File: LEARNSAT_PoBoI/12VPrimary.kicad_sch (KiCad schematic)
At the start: 17 parts, among them Q201 SI7164DP-T1-GE3, U201 INA219AIDCNR, U202 LTC4231IUD-2#TRPBF

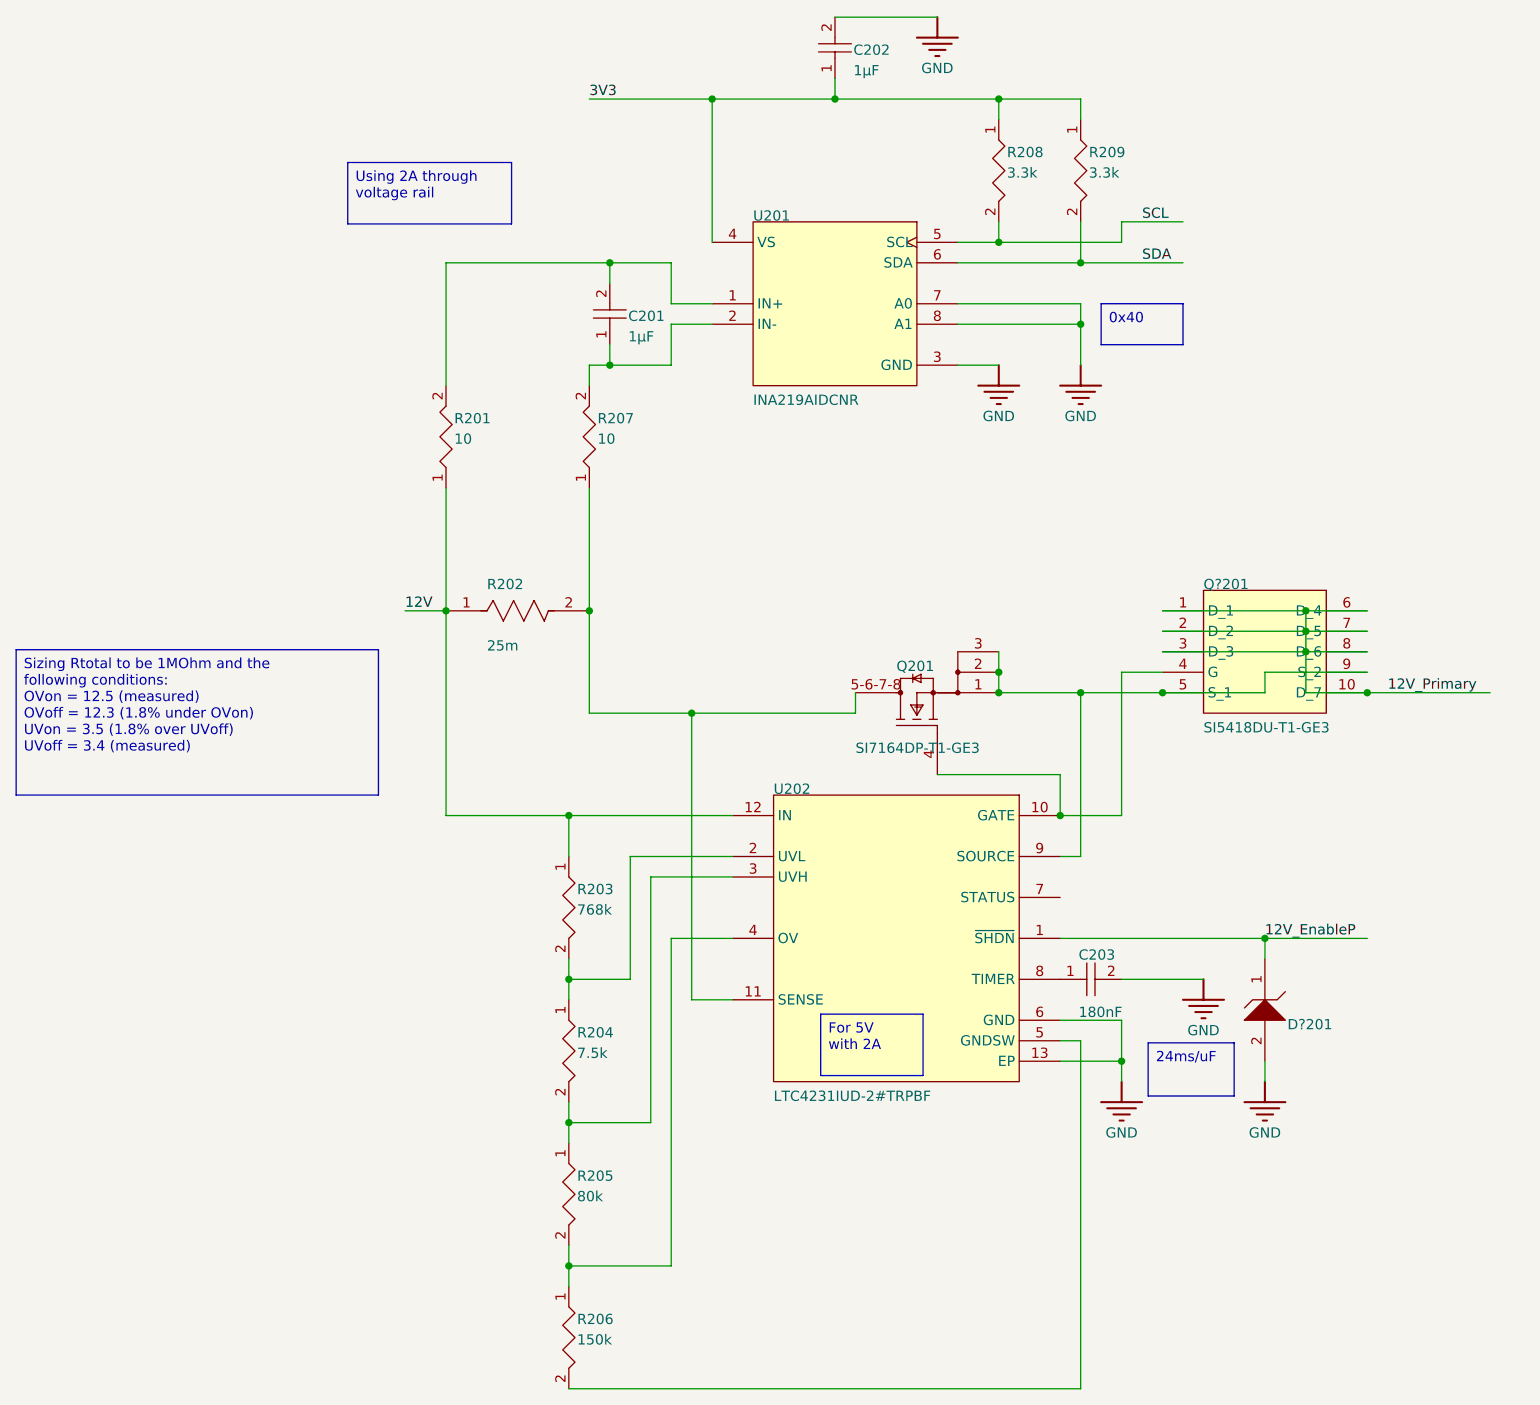
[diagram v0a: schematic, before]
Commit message: Add files via upload
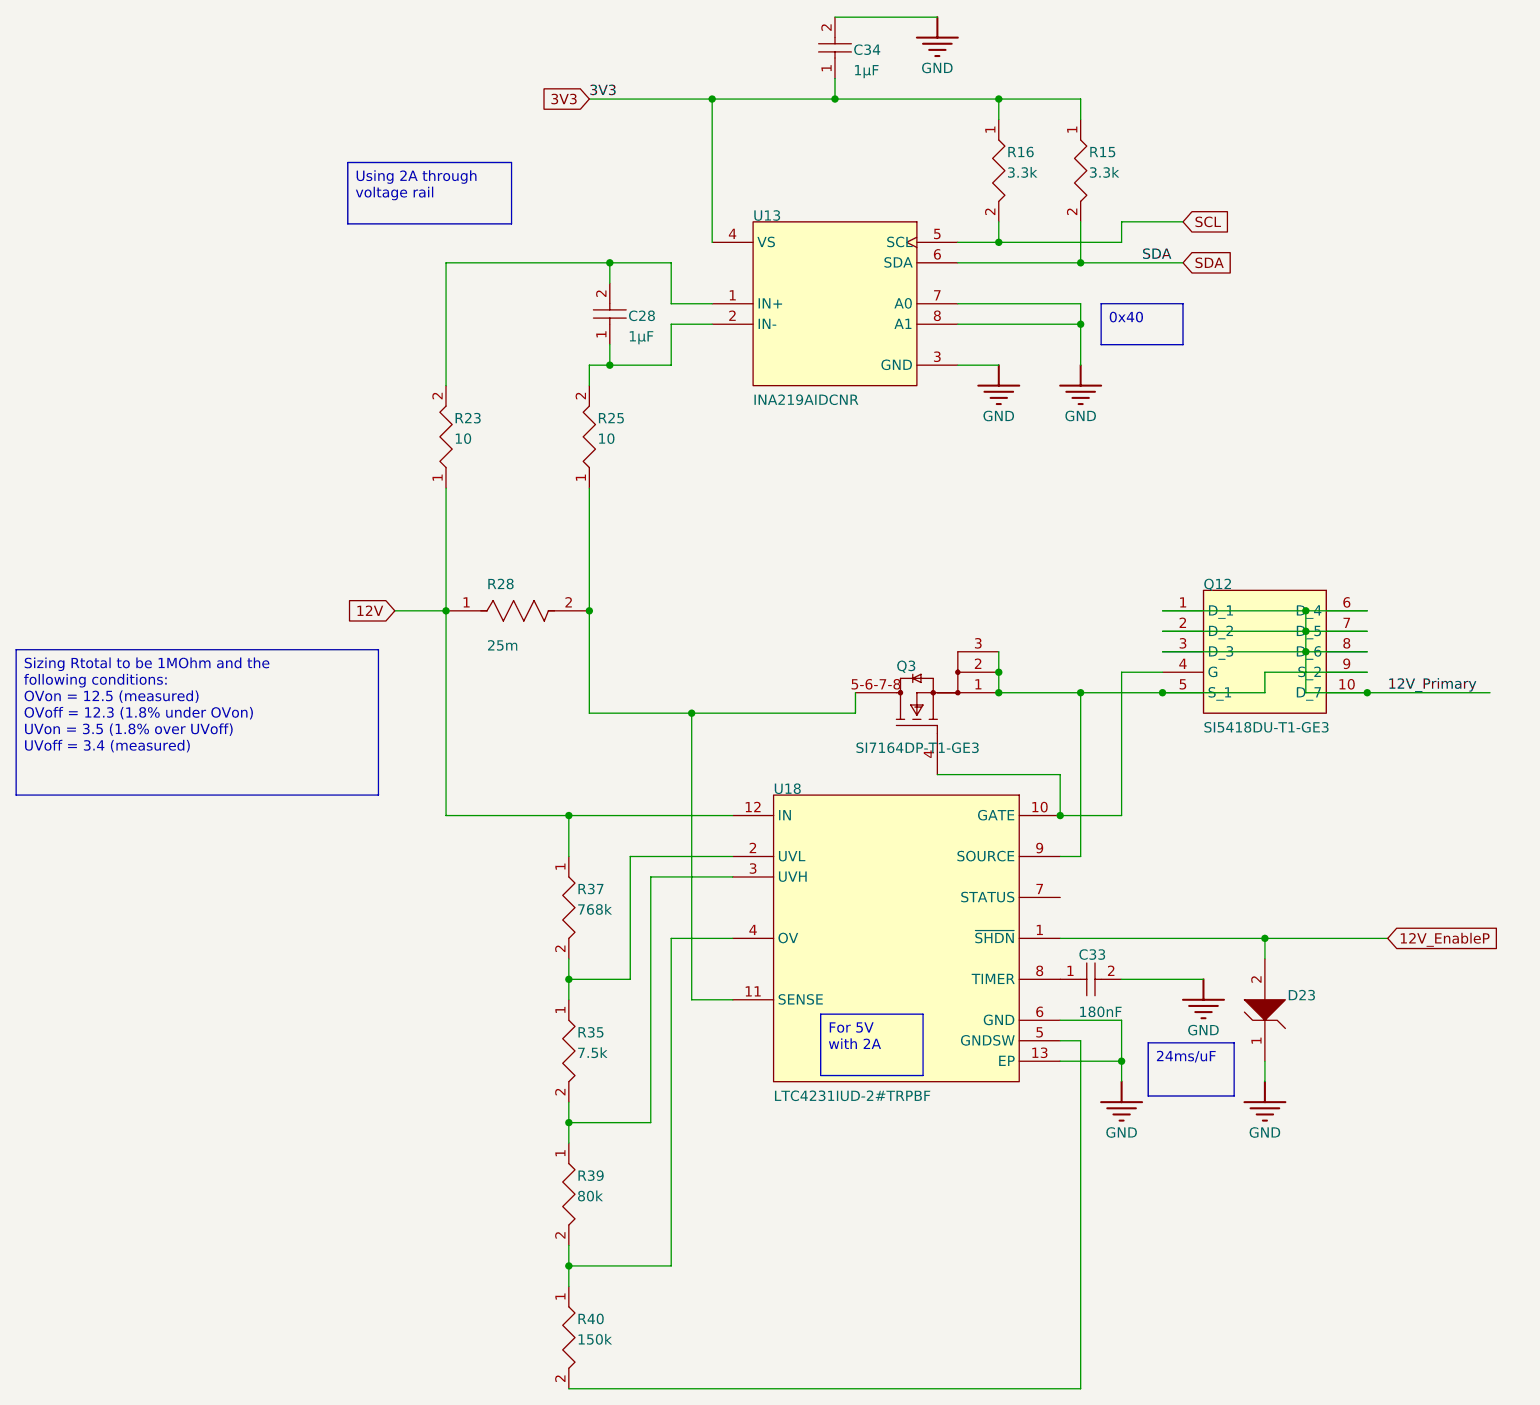
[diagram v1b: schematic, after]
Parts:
- C28: renamed from C201; footprint Capacitor_SMD:C_0603_1608Metric -> CAPC1608X90X40LL10T20
- C33: renamed from C203; footprint Capacitor_SMD:C_0805_2012Metric -> FP-C0805C-DN-IPC_A
- C34: renamed from C202; footprint Capacitor_SMD:C_0603_1608Metric -> CAPC1608X90X35ML15T15
- D23: renamed from D?201; footprint Diode_SMD:D_SOD-323 -> ONSC-SOD-323-2-477-02_V
- Q12: renamed from Q?201; footprint Package_SO:Vishay_PowerPAK_1212-8_Single -> SI5418DU-T1-GE3-Footprint-1
- Q3: renamed from Q201; footprint Package_SO:Vishay_PowerPAK_1212-8_Single -> Vishay_S17-0173-SINGLE_MFG
- R15: renamed from R209; footprint Resistor_SMD:R_1210_3225Metric -> FP-CRCW1210-e3-IPC_C
- R16: renamed from R208; footprint Resistor_SMD:R_1210_3225Metric -> FP-CRCW1210-e3-IPC_C
- R23: renamed from R201; footprint Resistor_SMD:R_0402_1005Metric -> RESC0402(1005)_L
- R25: renamed from R207; footprint Resistor_SMD:R_0402_1005Metric -> RESC0402(1005)_L
- R28: renamed from R202; footprint Resistor_SMD:R_1206_3216Metric -> FP-CSR1206-IPC_C
- R35: renamed from R204; footprint Resistor_SMD:R_1206_3216Metric -> FP-CRCW1206-e3-IPC_A
- R37: renamed from R203; footprint Resistor_SMD:R_0402_1005Metric -> RESC0402(1005)_L
- R39: renamed from R205; footprint Resistor_SMD:R_0603_1608Metric -> FP-PTN0603-IPC_B
- R40: renamed from R206; footprint Resistor_SMD:R_1206_3216Metric -> FP-RT1206-IPC_C
- U13: renamed from U201; footprint INA219AIDCNR:SOT65P280X145-8N -> FP-DCN0008A-IPC_A
- U18: renamed from U202; footprint LTC4231IUD-2_TRPBF:QFN50P300X300X80-13N -> FP-UD-12-05-08-1855-IPC_A
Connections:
- net 12V_EnableP: now also D23.2 (A); no longer D23.1 (K)
- net GND: now also D23.1 (K); no longer D23.2 (A)
